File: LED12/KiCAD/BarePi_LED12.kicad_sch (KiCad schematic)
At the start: 17 parts, among them J1 IN, J2 OUT, J3 WCH-LINK, U1 CH32V006E8R6

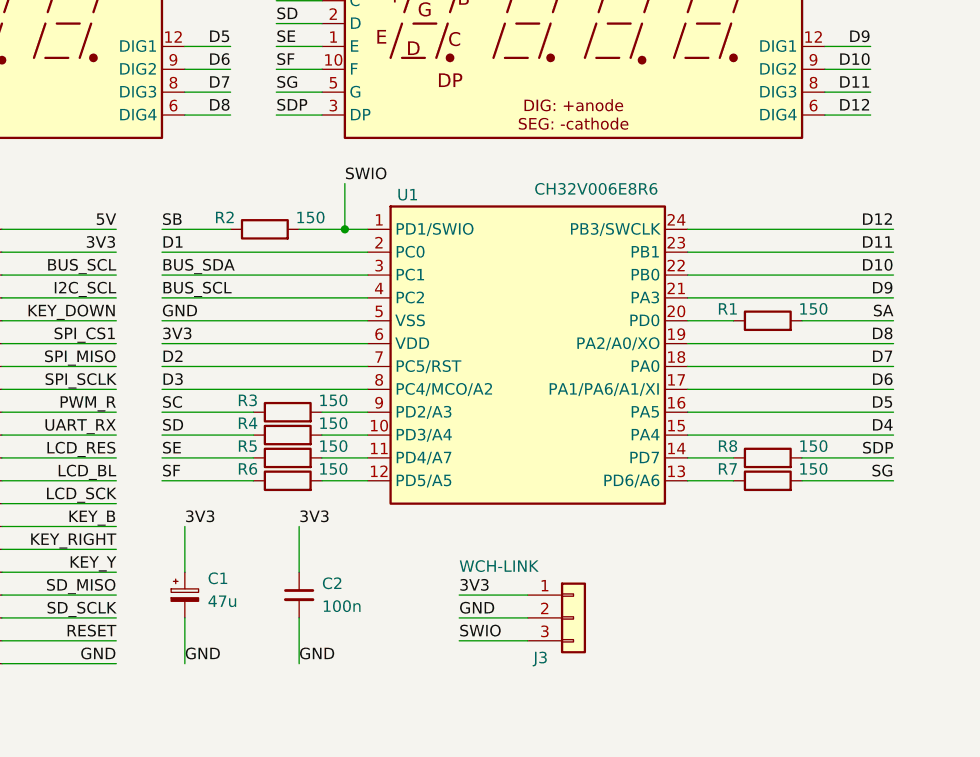
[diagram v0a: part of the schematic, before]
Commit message: init
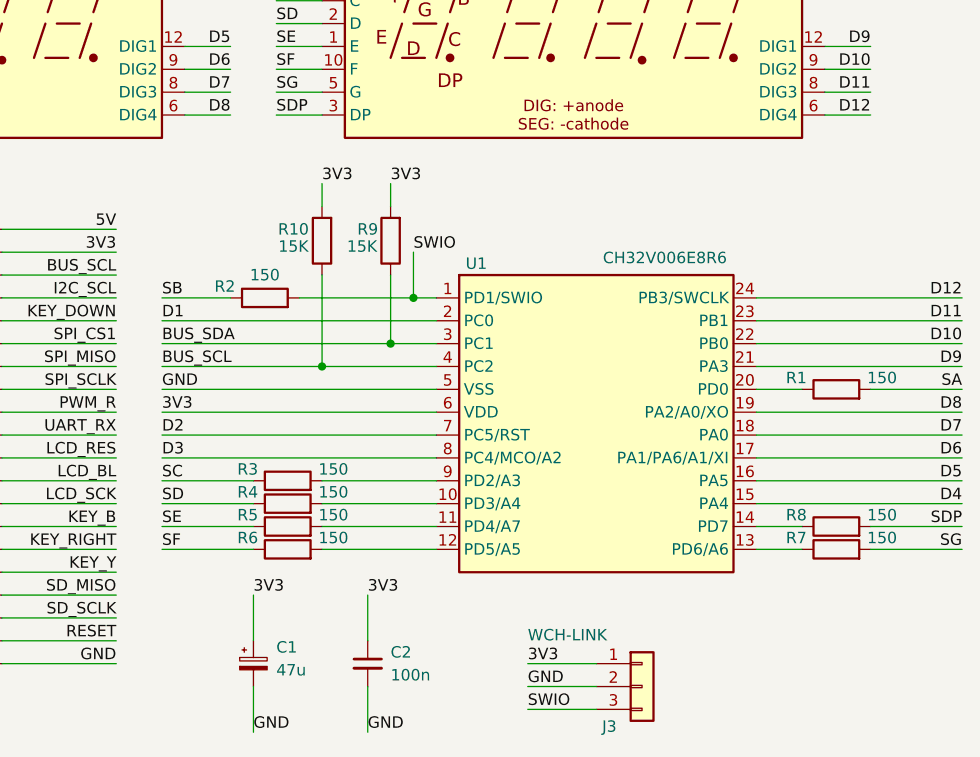
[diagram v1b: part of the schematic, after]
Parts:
- added R10, R9: 15K, Resistor_SMD:R_1206_3216Metric_Pad1.30x1.75mm_HandSolder, symbol Device:R
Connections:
- net 3V3: now also R10.2, R9.2
- net BUS_SCL: now also R10.1
- net BUS_SDA: now also R9.1
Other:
- moved on the sheet: C1, C2, J3, R1, R2, R3, R4, R5, R6, R7, R8, U1
